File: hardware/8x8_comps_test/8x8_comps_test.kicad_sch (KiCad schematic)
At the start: 8 parts

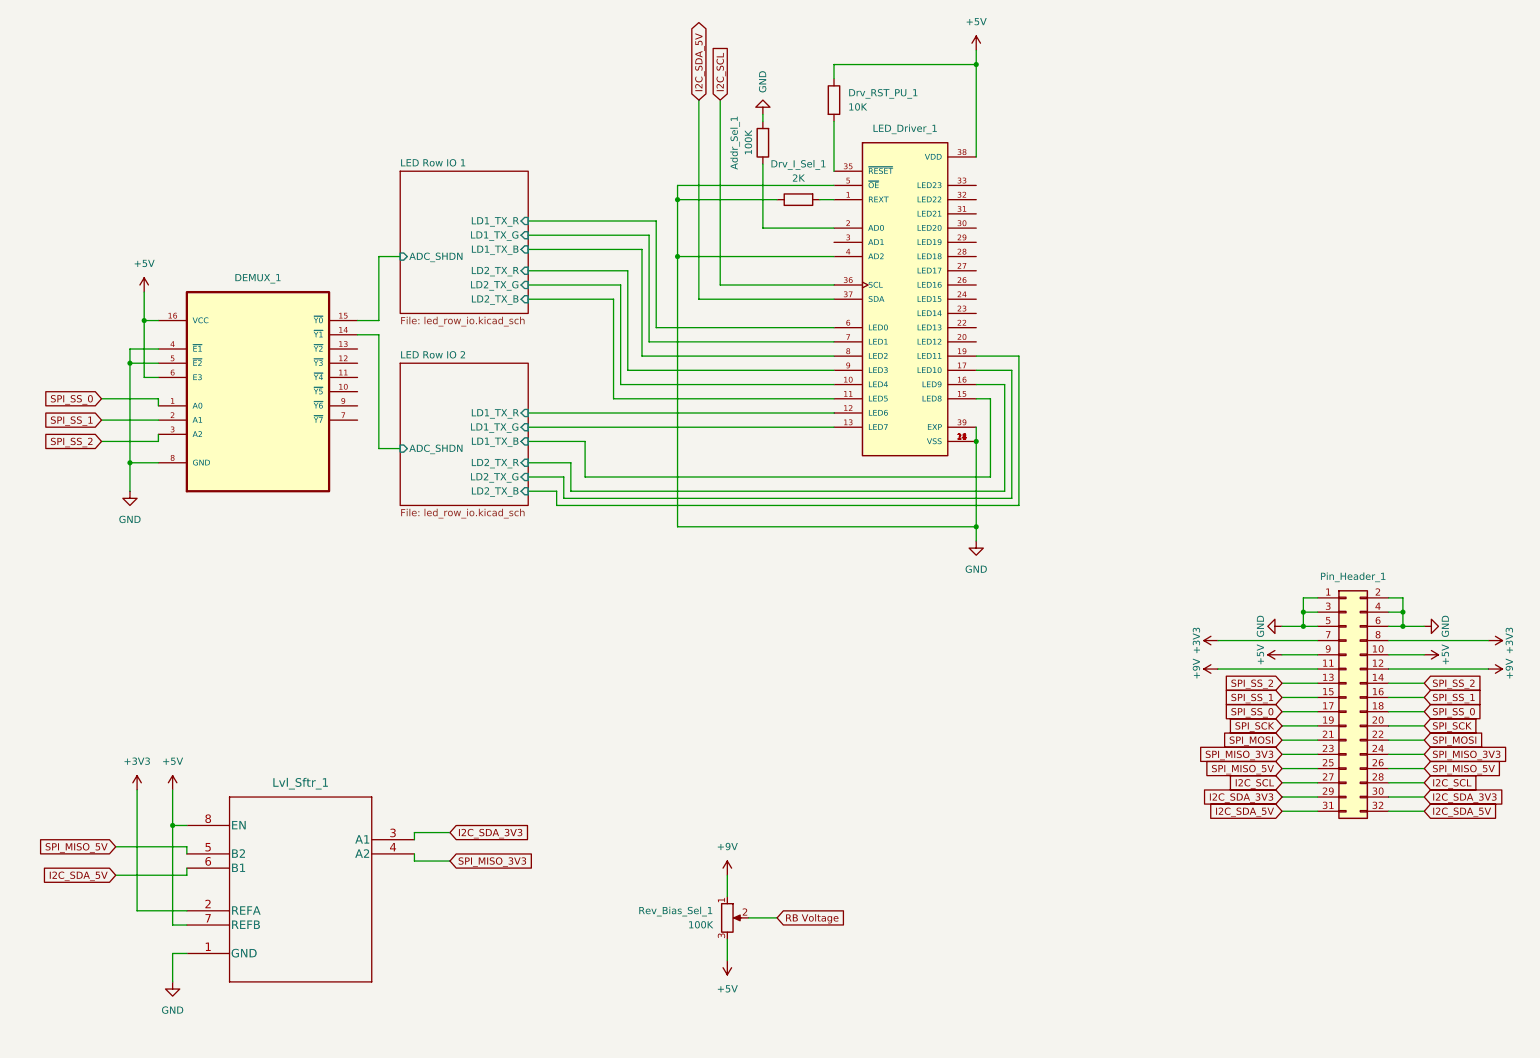
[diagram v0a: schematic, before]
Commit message: Updated PCB
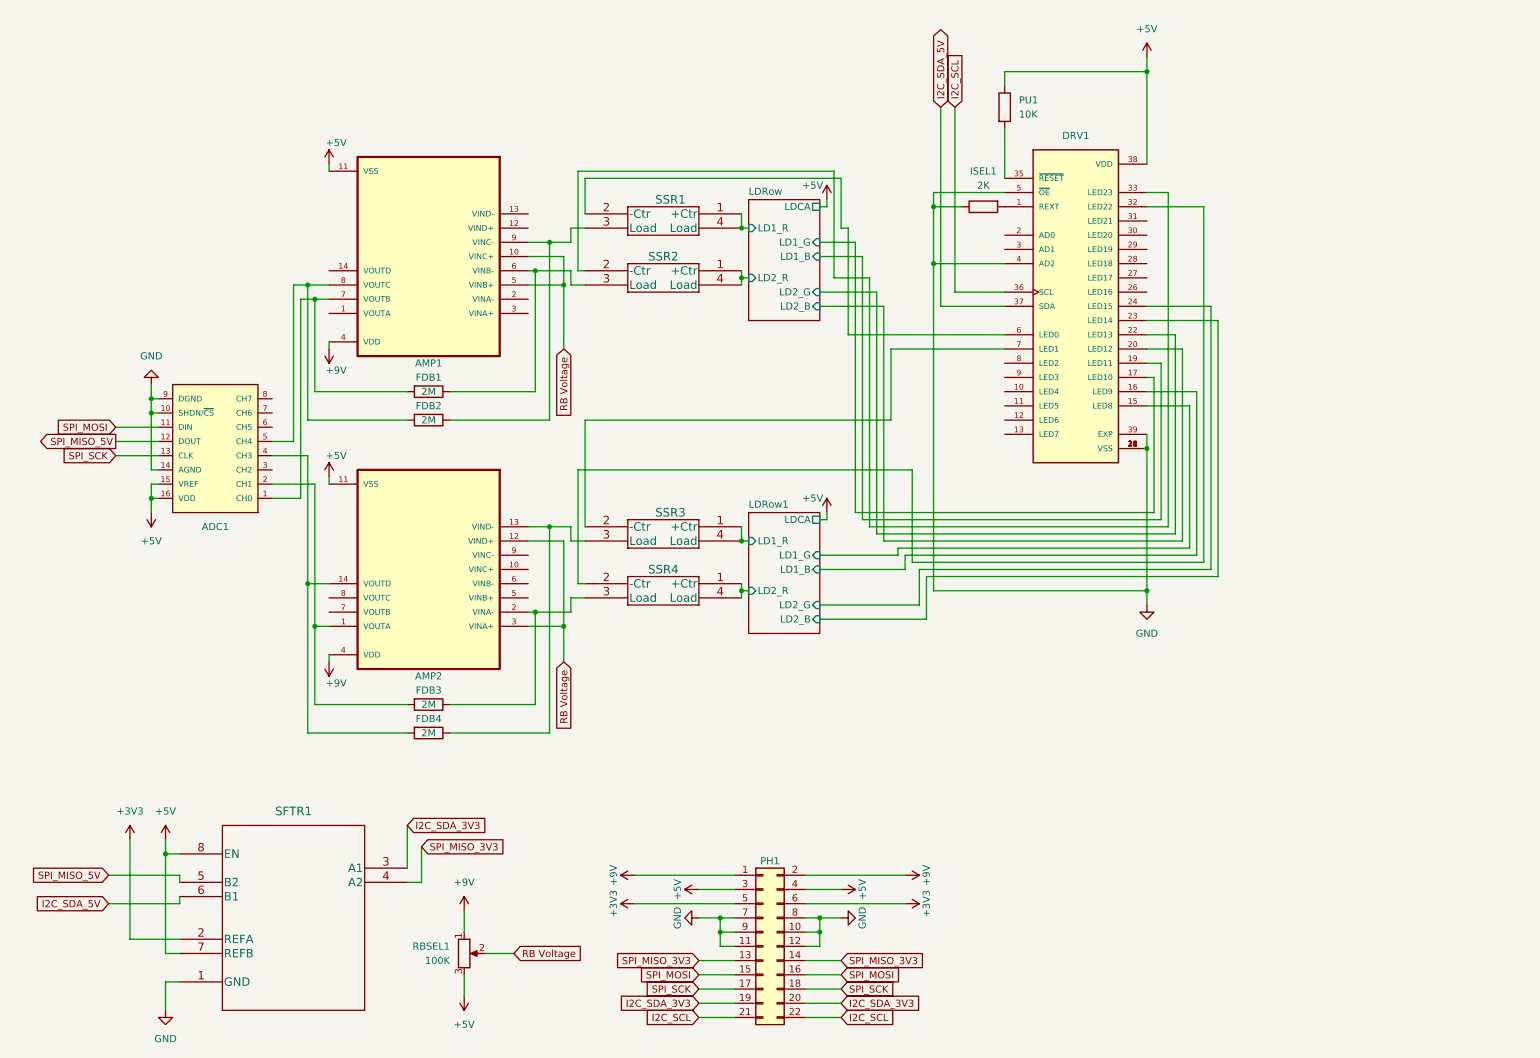
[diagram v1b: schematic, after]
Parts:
- removed Addr_Sel_1: 100K, Resistor_THT:R_Axial_DIN0207_L6.3mm_D2.5mm_P7.62mm_Horizontal, symbol Device:R
- removed DEMUX_1: 74HC138D-Q100,118, DEMUX:footprints, symbol DEMUX:74HC138D-Q100,118
- removed Pin_Header_1: Conn_02x16_Odd_Even, Connector_PinHeader_2.54mm:PinHeader_2x16_P2.54mm_Vertical, symbol Connector_Generic:Conn_02x16_Odd_Even
- added ADC1: MCU-MCP3008-I/P(DIP16-7.62MM), ADC:MCP3008-I&slash_P, symbol ADC:MCU-MCP3008-I{brace}slash}P(DIP16-7.62MM)
- added AMP1, AMP2: MCP619-I/SL, Op-Amp:footprints, symbol Op-Amp:MCP619-I{brace}slash}SL
- added FDB1, FDB2, FDB3, FDB4: 2M, Resistor - Through-Hole:footprints, symbol Device:R
- added PH1: Conn_02x11_Odd_Even, Connector_PinSocket_2.54mm:PinSocket_2x11_P2.54mm_Vertical, symbol Connector_Generic:Conn_02x11_Odd_Even
- added SSR1, SSR2, SSR3, SSR4: TLP417A-TP-F, SSR:footprints, symbol SSR:TLP4176ATP_F
- DRV1: renamed from LED_Driver_1; footprint SOP50P640X110-39N -> LED Driver:SOP50P640X110-39N
- ISEL1: renamed from Drv_I_Sel_1; footprint Resistor_THT:R_Axial_DIN0207_L6.3mm_D2.5mm_P7.62mm_Horizontal -> Resistor - Through-Hole:footprints
- PU1: renamed from Drv_RST_PU_1; footprint Resistor_THT:R_Axial_DIN0207_L6.3mm_D2.5mm_P7.62mm_Horizontal -> Resistor - Through-Hole:footprints
- renumbered Rev_Bias_Sel_1 to RBSEL1, Lvl_Sftr_1 to SFTR1
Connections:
- net +3V3: now also PH1.5 (Pin_5), PH1.6 (Pin_6)
- net +5V: now also ADC1.15 (VREF), ADC1.16 (VDD), AMP1.11 (VSS), AMP2.11 (VSS), PH1.3 (Pin_3), PH1.4 (Pin_4)
- net +9V: now also AMP1.4 (VDD), AMP2.4 (VDD), PH1.1 (Pin_1), PH1.2 (Pin_2)
- net GND: now also ADC1.10 (SHDN/~{CS}), ADC1.14 (AGND), ADC1.9 (DGND), PH1.10 (Pin_10), PH1.11 (Pin_11), PH1.12 (Pin_12), PH1.7 (Pin_7), PH1.8 (Pin_8), PH1.9 (Pin_9)
- net I2C_SCL: now also PH1.21 (Pin_21), PH1.22 (Pin_22)
- net I2C_SDA_3V3: now also PH1.19 (Pin_19), PH1.20 (Pin_20)
- net RB Voltage: now also AMP1.10 (VINC+), AMP1.5 (VINB+), AMP2.12 (VIND+), AMP2.3 (VINA+)
- net SPI_MISO_3V3: now also PH1.13 (Pin_13), PH1.14 (Pin_14)
- net SPI_MISO_5V: now also ADC1.12 (DOUT)
- net SPI_MOSI: now also ADC1.11 (DIN), PH1.15 (Pin_15), PH1.16 (Pin_16)
- net SPI_SCK: now also ADC1.13 (CLK), PH1.17 (Pin_17), PH1.18 (Pin_18)
- net LDRow/LD2_B: now reaches DRV1.20 (LED12)
- net LDRow/LD2_G: now reaches DRV1.22 (LED13)
- net LDRow1/LD2_B: now reaches DRV1.23 (LED14)
- net LDRow1/LD2_G: now reaches DRV1.24 (LED15)
- net at DRV1.32 (LED22): now also SSR4.2 (-Ctr)
- net at DRV1.33 (LED23): now also SSR2.2 (-Ctr)
- net LED Row IO 1/LD1_TX_B: no longer names the net of DRV1.8 (LED2)
- net LED Row IO 1/LD1_TX_G: no longer names the net of DRV1.7 (LED1)
- net LED Row IO 1/LD1_TX_G: now also SSR3.2 (-Ctr)
- net LED Row IO 1/LD1_TX_R: no longer names the net of DRV1.6 (LED0)
- net LED Row IO 1/LD1_TX_R: now also SSR1.2 (-Ctr)
- net LED Row IO 1/LD2_TX_B: no longer names the net of DRV1.11 (LED5)
- net LED Row IO 1/LD2_TX_G: no longer names the net of DRV1.10 (LED4)
- net LED Row IO 1/LD2_TX_R: no longer names the net of DRV1.9 (LED3)
- net LED Row IO 2/LD1_TX_B renamed LDRow1/LD1_G
- net LED Row IO 2/LD1_TX_G: no longer names the net of DRV1.13 (LED7)
- net LED Row IO 2/LD1_TX_R: no longer names the net of DRV1.12 (LED6)
- net LED Row IO 2/LD2_TX_B renamed LDRow/LD1_B
- net LED Row IO 2/LD2_TX_G renamed LDRow/LD1_G
- net LED Row IO 2/LD2_TX_R renamed LDRow1/LD1_B
- new net: AMP1.6 (VINB-), FDB1.1, SSR2.3 (Load)
- new net: ADC1.1 (CH0), AMP1.7 (VOUTB), FDB1.2
- new net: ADC1.2 (CH1), AMP2.1 (VOUTA), FDB3.2
- new net: ADC1.4 (CH3), AMP2.14 (VOUTD), FDB4.2
- new net: ADC1.5 (CH4), AMP1.8 (VOUTC), FDB2.2
- new net: AMP2.13 (VIND-), FDB4.1, SSR3.3 (Load)
- new net: AMP1.9 (VINC-), FDB2.1, SSR1.3 (Load)
- new net: AMP2.2 (VINA-), FDB3.1, SSR4.3 (Load)
- new net LDRow/LD1_R: SSR1.1 (+Ctr), SSR1.4 (Load)
- new net LDRow/LD2_R: SSR2.1 (+Ctr), SSR2.4 (Load)
- new net LDRow1/LD1_R: SSR3.1 (+Ctr), SSR3.4 (Load)
- new net LDRow1/LD2_R: SSR4.1 (+Ctr), SSR4.4 (Load)
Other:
- removed sheet LED Row IO 1
- removed sheet LED Row IO 2
- added sheet LDRow (led_row.kicad_sch)
- added sheet LDRow1 (led_row.kicad_sch)
- moved on the sheet: DRV1, ISEL1, PU1, RBSEL1, SFTR1
